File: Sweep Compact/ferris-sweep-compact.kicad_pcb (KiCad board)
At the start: 2 copper layers, 107.2 x 86.9 mm, 21 parts, among them J1 MJ-4PP-9, SW10 SW_PUSH, SW11 SW_PUSH, SW12 SW_PUSH, SW14 SW_PUSH, SW15 SW_PUSH, SW16 SW_PUSH, SW17 SW_PUSH, SW18 SW_PUSH, SW2 SW_PUSH, SW20 SW_PUSH, SW21 SW_PUSH, SW3 SW_PUSH, SW4 SW_PUSH, SW5 SW_PUSH, SW6 SW_PUSH, SW8 SW_PUSH, SW9 SW_PUSH, U1 ProMicro

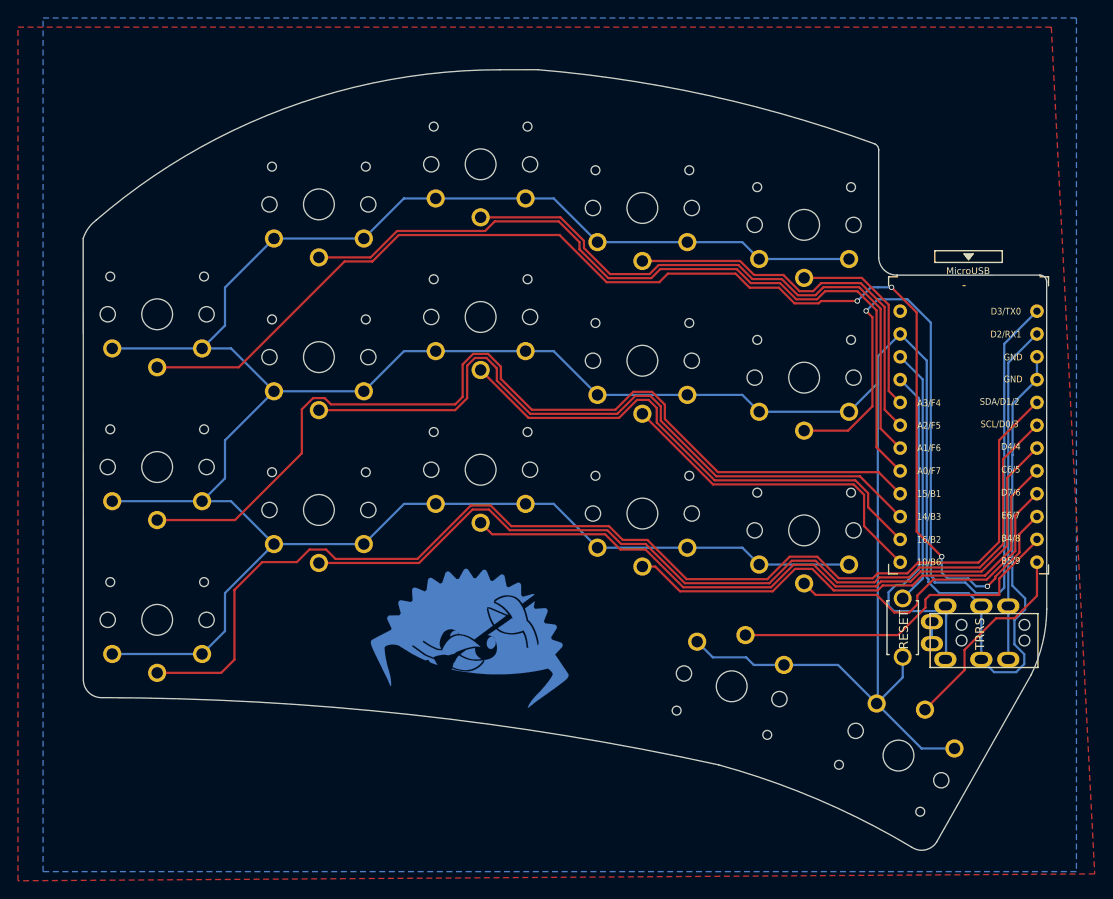
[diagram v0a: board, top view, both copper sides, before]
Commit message: update stagger
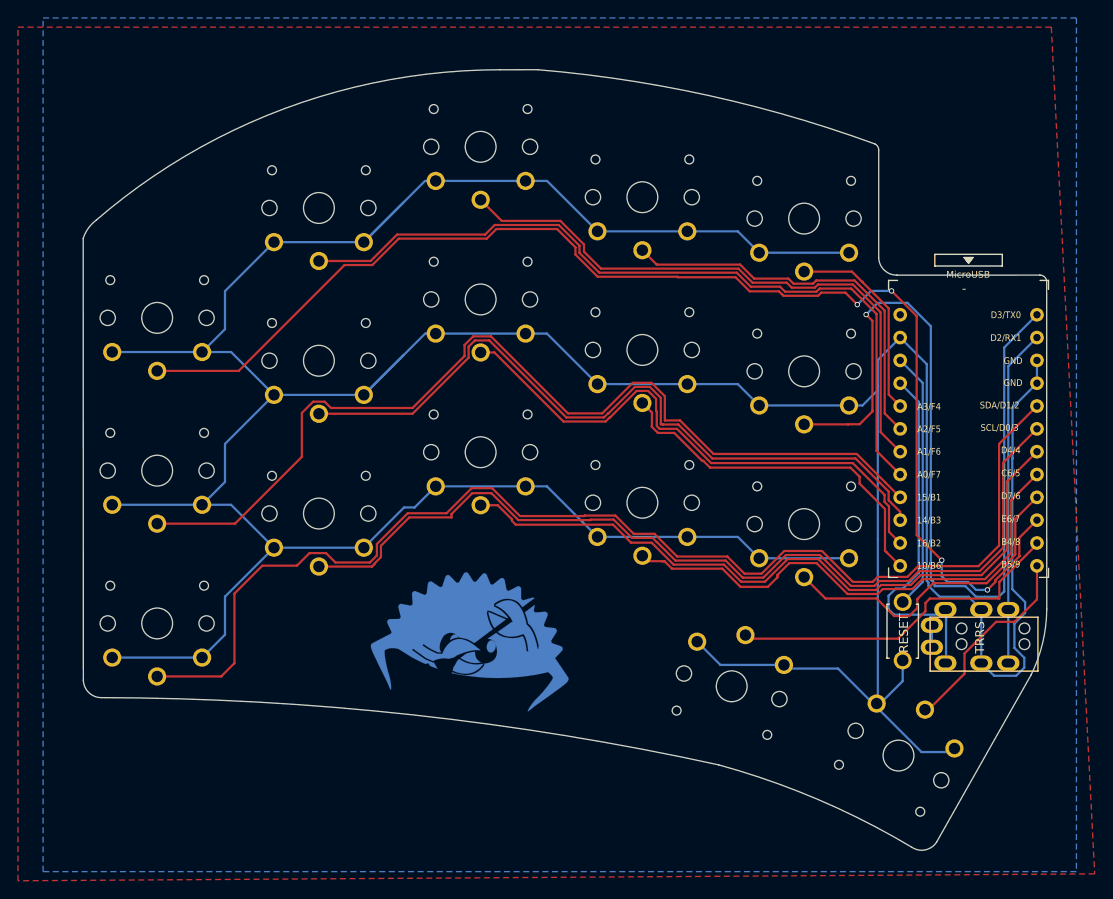
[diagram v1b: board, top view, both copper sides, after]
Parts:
- moved SW10 1.95 mm to (80.0, 40.7)
- moved SW16 1.95 mm to (80.0, 57.7)
- moved SW4 1.95 mm to (80.0, 23.7)
- moved SW17 1.20 mm to (98.0, 63.3)
- moved SW5 1.20 mm to (98.0, 29.3)
- moved SW11 1.20 mm to (98.0, 46.3)
- moved SW12 0.70 mm to (116.0, 48.7)
- moved SW18 0.70 mm to (116.0, 65.7)
- moved SW6 0.70 mm to (116.0, 31.7)
- moved RSW1 0.40 mm to (127.0, 77.6)
- moved SW14 0.40 mm to (44.0, 76.8)
- moved SW15 0.40 mm to (62.0, 64.5)
- moved SW2 0.40 mm to (44.0, 42.8)
- moved SW8 0.40 mm to (44.0, 59.8)
- moved SW3 0.40 mm to (62.0, 30.5)
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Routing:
- net GND: track 473.9 -> 490.3 mm
- net Net-(U1-Pad14): track 58.0 -> 62.1 mm
- net SCL: track 100.6 -> 103.5 mm
- net col5: track 79.9 -> 82.7 mm
- net SDA: track 131.2 -> 133.9 mm
- net Net-(U1-Pad13): track 37.6 -> 40.3 mm
- net col4: track 105.7 -> 107.3 mm
- net row1: track 56.0 -> 57.5 mm
- net col3: track 88.8 -> 87.5 mm
- net row0: track 77.7 -> 78.8 mm
- net row3: track 142.4 -> 143.0 mm
- net col0: track 22.1 -> 22.6 mm
